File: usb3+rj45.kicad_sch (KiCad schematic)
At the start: 67 parts, among them J1 RJE361882415, T1 Choke_SRF2012A-801Y, T2 Choke_SRF2012A-801Y, T3 Choke_SRF2012A-801Y, T4 Choke_SRF2012A-801Y, T5 Trans_SM453229-381N7Y, T6 Trans_SM453229-381N7Y, T7 Trans_SM453229-381N7Y, T8 Trans_SM453229-381N7Y, U1 ESD204DQAR, U2 ESD204DQAR, U3 AP22615A_TSOT26, U4 AP22615A_TSOT26

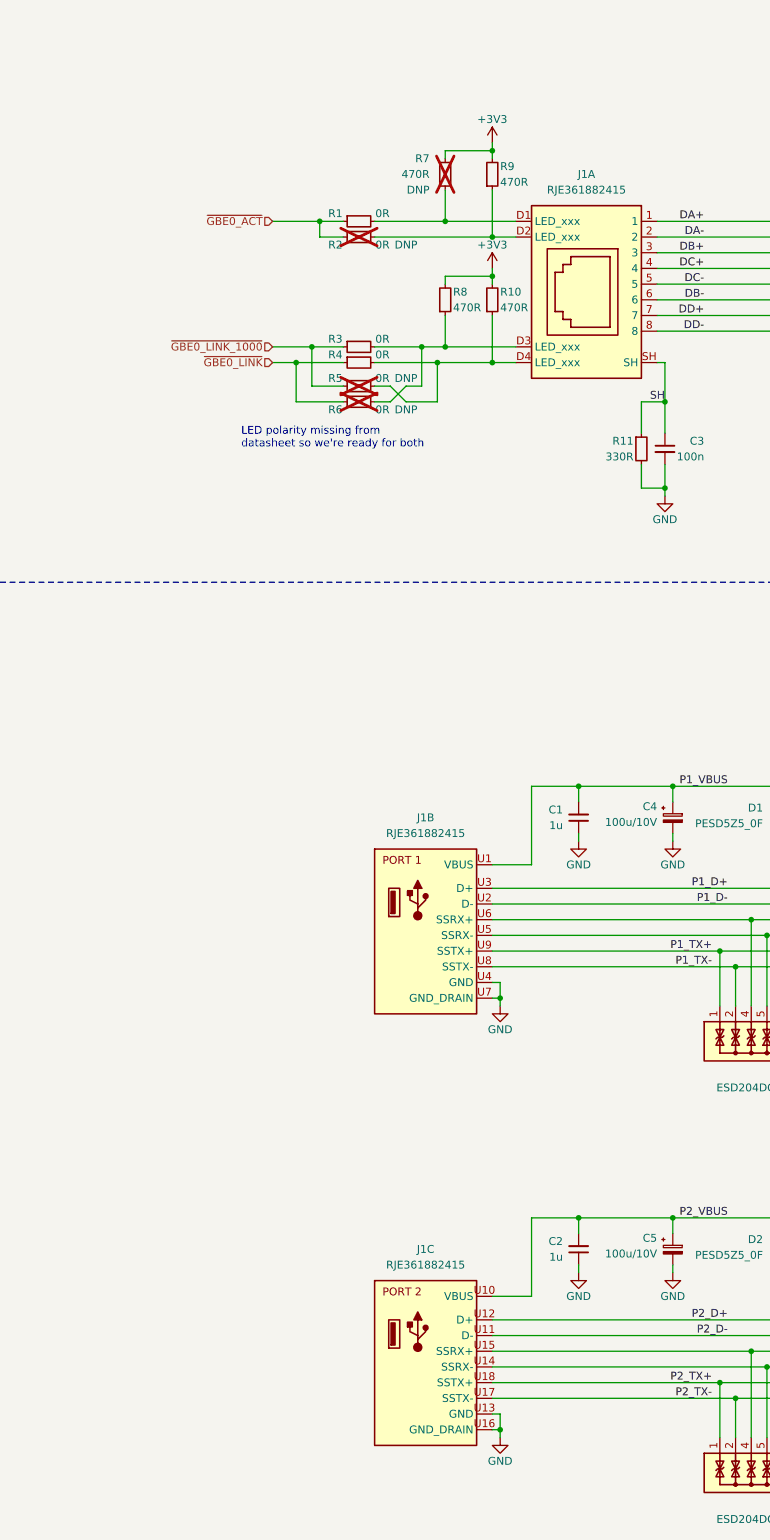
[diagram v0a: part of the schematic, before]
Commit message: Update symbols from the library
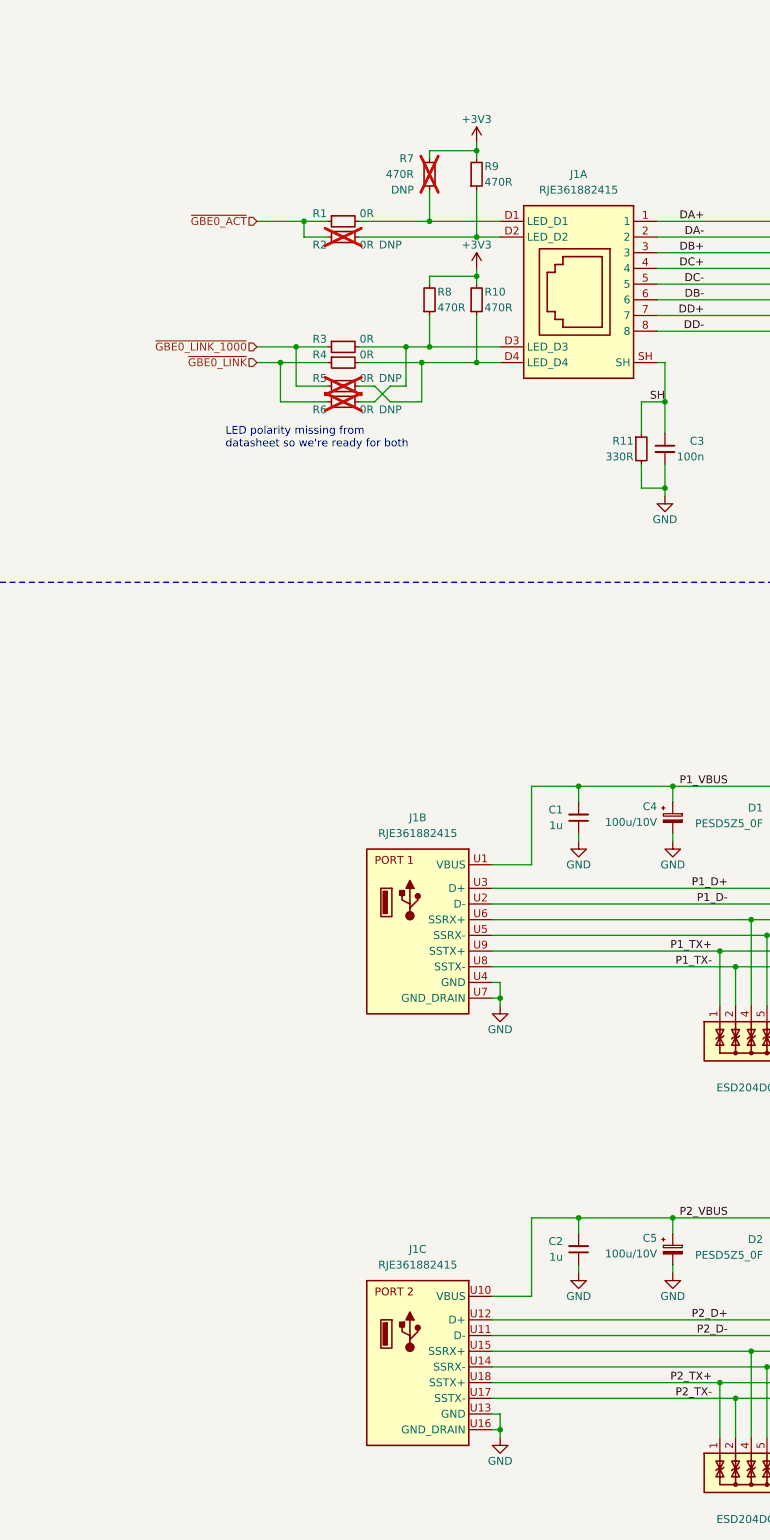
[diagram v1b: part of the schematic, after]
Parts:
- J1: footprint (none) -> antmicro-footprints:RJ45_RJE361882415; Author (none) -> Antmicro; License (none) -> Apache-2.0
- T1, T2, T3, T4: footprint (none) -> antmicro-footprints:Choke_0805_2012Metric
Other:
- moved on the sheet: J1A, J1B, J1C, R1, R10, R2, R3, R4, R5, R6, R7, R8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
